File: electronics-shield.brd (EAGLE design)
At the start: 85 x 56 mm, 83 parts, among them IC1 MCP1703CB, Q1 8 MHz, Q2 MOSFET-PCHANNELSMD, U1 TLE9201SGAUMA1, U2 TLE9201SGAUMA1, U3 TLE9201SGAUMA1, U4 TLE9201SGAUMA1, U5 STM32F051C8T, U6 SN74LVC4245APWR, U7 SN74LVC4245APWR, U8 24LC256

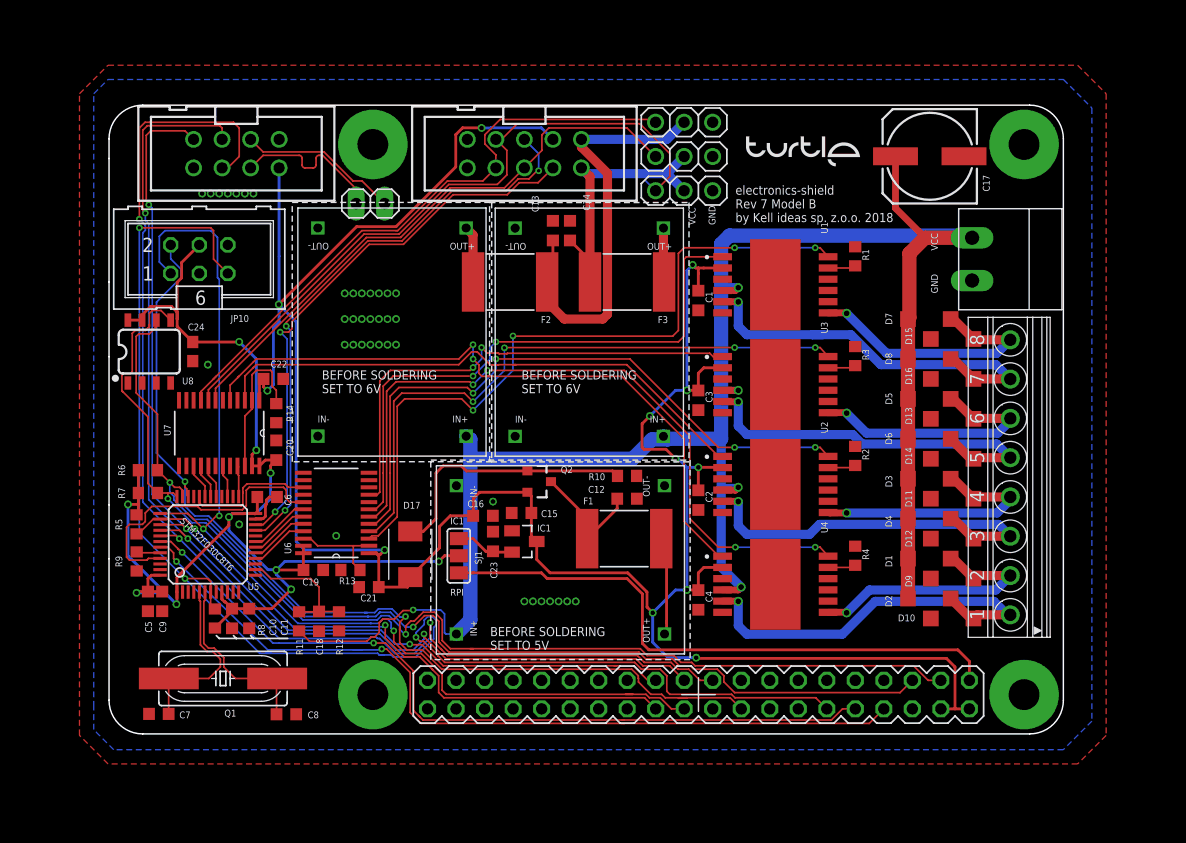
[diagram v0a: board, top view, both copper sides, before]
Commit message: changed base for 7.c
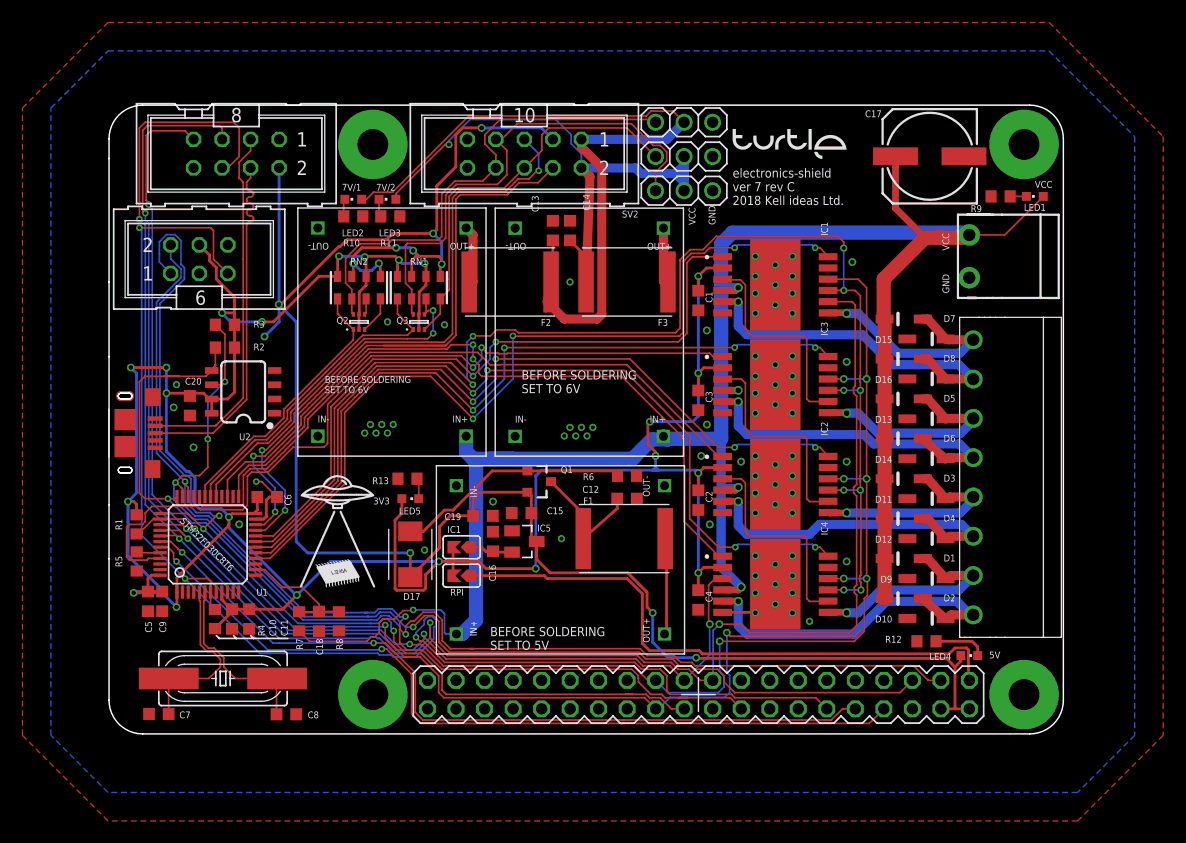
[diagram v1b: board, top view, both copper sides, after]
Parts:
- removed C21, C22, C23: 100n, resistor:C0603K
- removed C24: 0.1uF, rcl:C0603
- removed JP10: gniazdo IDC męskie 6pin proste, con-harting-ml:ML6
- removed JP4: Listwa kołkowa 2.54mm prosta 1x3 (3pin), Synergiczne:1X03
- removed JP5: Listwa stykowa 2.54mm prosta 2x20 (40-pin), wydłużona, RASPBERRY_PI_Bplus-eagle5:2X20
- removed JP6: gniazdo IDC męskie 10pin proste, con-3m:PAK100/2500-10
- removed JP7: gniazdo IDC męskie 8pin proste, Simplex-Connectors:PAK100/2500-10
- removed JP8: Listwa zaciskowa rozłączalna 3.81mm 2pin kątowe 90° gniazdo, con-phoenix-381_l:MC2
- removed JP9: Listwa zaciskowa rozłączalna 3.50mm 8pin kątowe 90° gniazdo, con-phoenix-350:1751303
- removed PCB2, PCB3: Moduł przetwornicy DC-DC Step-down 4.5..28V --- regulowane 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, Kell Ideas:MP1584_MODULE
- removed R14: 10k, resistor:R0603
- removed U5: STM32F051C8T, STM32F030:LQFP48
- removed U6, U7: SN74LVC4245APWR, Texas Instruments_By_element14_Batch_1:SOP65P640X120-24N
- removed U8: 24LC256, SparkFun-IC-Memory:SO08
- added $3_0_$_2018-08-14_21-12-08, $3_1_$_2018-08-14_21-12-08, $3_2_$_2018-08-14_21-12-08: Moduł przetwornicy DC-DC Step-down 4.5..28V --- regulowane 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, Kell Ideas:DC-BRICK
- added IC2: TLE9201SG, Kell Ideas:PG-DSO-12-9
- added IC5: LINEAR_MCP1703CB, electronics-shield:LINEAR_SOT23
- added J1: USB-MICRO-B, Kell Ideas:USB-MICRO-B
- added LED1, LED2, LED3, LED4, LED5: LEDCHIPLED_0603, audio amplifier example:CHIPLED_0603
- added Q3: ON-SEMICONDUCTOR---NTZD3154NT1G_ON_SEMICONDUCTOR_NTZD3154NT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, electronics-shield:ON-SEMICONDUCTOR---NTZD3154NT1G_ON_SEMICONDUCTOR_NTZD3154NT1G_0
- added RN1, RN2: 1k, SparkFun-Resistors:0805-ARV
- added SJ2: (no value), Kell Ideas:SJ
- added SV1: gniazdo IDC męskie 6pin proste, Kell Ideas:ML6
- added SV2: (no value), Kell Ideas:ML10
- added SV3: ML8, Kell Ideas:ML8
- added X1: CONNECTOR_PHOENIX_3.81, Kell Ideas:3.81MM_2PIN
- added X2: Listwa zaciskowa rozłączalna 3.50mm 8pin kątowe 90° gniazdo, Kell Ideas:3.5MM_8PIN
- added Y1: 8 MHz, Kell Ideas:HC49UP
- C1, C10, C11, C12, C13, C14, C15, C16, C18, C19, C2, C3, C4, C5, C6, C7, C8, C9: device resistor:C0603K -> Kell Ideas:C0603K
- C17: device resistor:153CLV-0807 -> Kell Ideas:FI8_6.2
- C20: value 100n -> 0.1uF; device resistor:C0603K -> Kell Ideas:C0603K
- D1, D10, D11, D12, D13, D14, D15, D16, D2, D3, D4, D5, D6, D7, D8, D9: device diode:SOD123 -> Kell Ideas:SOD123
- D17: device diode:SMBJ -> Kell Ideas:SMBJ
- F1, F2, F3: device polyfuse-smd_10:2920L -> Kell Ideas:FUSC7351X125
- IC1: value MCP1703CB -> TLE9201SG; device linear:SOT23 -> Kell Ideas:PG-DSO-12-9
- IC3, IC4: value TLE9201SGAUMA1 -> TLE9201SG
- JP1: value Listwa kołkowa 2.54mm prosta 1x2 (2pin) -> Listwa kołkowa 2.54mm prosta 1x3 (3pin); device pinhead:1X02 -> Kell Ideas:1X03_ROUND_DNP
- JP2, JP3: device Synergiczne:1X03 -> Kell Ideas:1X03_ROUND_DNP
- PCB1: value Moduł przetwornicy DC-DC Step-down 4.5..28V --- regulowane 0.8..20V MP1584 -> Listwa stykowa 2.54mm prosta 2x20 (40-pin), wydłużona; device Kell Ideas:MP1584_MODULE -> Kell Ideas:RASPBERRY_PI_B+_CONNECTOR
- Q1: value 8 MHz -> USER-SUBMITTED_MOSFET-PCHANNELSMD; device crystal:HC49UP -> electronics-shield:USER-SUBMITTED_SOT23-3
- Q2: value MOSFET-PCHANNELSMD -> ON-SEMICONDUCTOR---NTZD3154NT1G_ON_SEMICONDUCTOR_NTZD3154NT1GON_SEMICONDUCTOR_NTZD3154NT1G_0_0; device User-Submitted:SOT23-3 -> electronics-shield:ON-SEMICONDUCTOR---NTZD3154NT1G_ON_SEMICONDUCTOR_NTZD3154NT1G_0
- R1, R4: device rcl:R0603 -> Kell Ideas:R0603
- R10: value 100k -> 330; device rcl:R0603 -> Kell Ideas:R0603
- R11: value 10k -> 330; device resistor:R0603 -> Kell Ideas:R0603
- R12: value 1k -> 200; device resistor:R0603 -> Kell Ideas:R0603
- R13: value 10k -> 200; device resistor:R0603 -> Kell Ideas:R0603
- R2, R3: value 10k -> 4k7; device rcl:R0603 -> Kell Ideas:R0603
- R5: device resistor:R0603 -> Kell Ideas:R0603
- R6: value 4k7 -> 100k; device resistor:R0603 -> Kell Ideas:R0603
- R7: value 4k7 -> 10k; device resistor:R0603 -> Kell Ideas:R0603
- R8: value 10k -> 1k; device resistor:R0603 -> Kell Ideas:R0603
- R9: value 10k -> 1.5k; device resistor:R0603 -> Kell Ideas:R0603
- SJ1: value Zworka cynowa -> (none); device jumper:SJ_2 -> Kell Ideas:SJ
- U1: value TLE9201SGAUMA1 -> STM32F0XX8T; device Kell Ideas:PG-DSO-12-9 -> Kell Ideas:LQFP48
- U2: value TLE9201SGAUMA1 -> EEPROM-I2C; device Kell Ideas:PG-DSO-12-9 -> Kell Ideas:SO-08
- moved R9 83.5 mm to (79.5, 48.0), turned to 180 degrees
- moved PCB1 74.2 mm to (85.1, 56.1), turned to 180 degrees
- moved R1 68.3 mm to (2.54, 18.8), turned to 90 degrees
- moved R4 57.3 mm to (9.53, 10.4)
- moved R2 57.0 mm to (10.4, 34.5), turned to 0 degrees
- moved R3 56.2 mm to (10.4, 36.6), turned to 0 degrees
- moved U1 55.6 mm to (8.89, 17.0), turned to 0 degrees
- moved R12 52.4 mm to (72.9, 8.38), turned to 180 degrees
- moved U2 48.1 mm to (12.0, 30.6), turned to 90 degrees
- moved R6 42.7 mm to (46.2, 23.1)
- moved R11 37.0 mm to (25.1, 46.2), turned to 0 degrees
- moved R10 33.6 mm to (21.8, 46.2), turned to 0 degrees
- moved Q1 33.1 mm to (38.4, 22.6), turned to 270 degrees
- moved IC1 32.0 mm to (59.4, 40.1)
- moved JP1 28.3 mm to (51.3, 51.6)
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- renumbered U3 to IC3, U4 to IC4
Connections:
- removed net EN1_UC: U5.16, U6.21
- removed net EN2_UC: U5.17, U6.20
- removed net EN3_UC: U5.18, U6.19
- removed net EN4_UC: U5.19, U6.18
- removed net IN11_UC: U5.45, U6.17
- removed net IN12: U6.8
- removed net IN12_UC: U6.16
- removed net IN21_UC: U5.32, U6.15
- removed net IN22: U6.10
- removed net IN22_UC: U6.14
- removed net IN31_UC: U5.25, U7.21
- removed net IN32: U7.4
- removed net IN32_UC: U7.20
- removed net IN41_UC: U5.27, U7.19
- removed net IN42: U7.6
- removed net IN42_UC: U7.18
- removed net U5_DIS: R1.2, U1.11
- removed net U6_DIS: R2.2, U2.11
- removed net U7_DIS: IC3.11, R3.2
- removed net U8_DIS: IC4.11, R4.2
- new net N$14: Q2.4, RN2.3
- new net N$16: Q2.3, RN2.4
- new net N$5: LED5.C, R13.1
- new net SO1-SI3: IC1.3, IC3.8
- new net SO2-SI4: IC2.3, IC4.8
- new net SO3-SI2: IC2.8, IC3.3
- new net TLE_NSS: IC1.9, IC2.9, IC3.9, IC4.9, U1.20
- net +3V3: now also C1.1, C2.1, C3.1, C4.1, IC1.2, IC2.2, IC3.2, IC4.2, LED5.A, Q2.2, Q2.5, Q3.2, Q3.5, R1.2, R2.2, R3.2, R4.2, RN1.6, RN1.8, RN2.6, RN2.8, SJ1.1, SJ2.1, SV1.4, U1.1, U1.24, U1.48, U1.9, U2.7, U2.8; no longer C19.1, C24.1, JP10.4, R5.2, R6.2, R7.2, R8.2, SJ1.2, U5.1, U5.24, U5.48, U5.9, U6.23, U6.24, U7.23, U7.24, U8.7, U8.8
- net +5V: now also C19.1, IC5.3, LED4.A, PCB1.2, PCB1.4, Q1.2, RN1.5, RN1.7, RN2.5, RN2.7, SV2.3, SV3.2; no longer C1.1, C2.1, C21.1, C22.1, C23.1, C3.1, C4.1, IC1.3, IC3.2, IC4.2, JP5.2, JP5.4, JP6.3, JP7.2, Q2.2, U1.2, U2.2, U6.1, U7.1
- net +5V_RAW: now also $3_0_$_2018-08-14_21-12-08.OUT1+1; no longer PCB1.OUT1+1
- net +7V/1: now also JP3.2, LED2.A, SV2.1; no longer JP4.2, JP6.1
- net +7V/1_RAW: now also $3_1_$_2018-08-14_21-12-08.OUT1+1; no longer PCB2.OUT1+1
- net +7V/2: now also JP1.2, LED3.A, SV2.2; no longer JP3.2, JP6.2
- net +7V/2_RAW: now also $3_2_$_2018-08-14_21-12-08.OUT1+1; no longer PCB3.OUT1+1
- net 3V3: now also PCB1.17; no longer JP5.17
- net 3V3_RPI: now also PCB1.1, SJ2.2; no longer JP5.1, SJ1.3
- net 3V3_STABILIZED: now also IC5.2, SJ1.2; no longer IC1.2, SJ1.1
- net 5V_NOT_TRIMMED: now also Q1.3; no longer Q2.3
- net BAT_MEAS: now also R7.1, R8.2, U1.14; no longer R11.1, R12.2, U5.14
- net BOOT0: now also R5.2, U1.44; no longer R9.2, U5.44
- net D1-R3: now also Q1.1, R6.2; no longer Q2.1, R10.2
- net DATA_N: now also J1.D-, SV3.3; no longer JP1.2, JP7.3
- net DATA_P: now also J1.D+, SV3.4; no longer JP1.1, JP7.4
- net EN1: now also IC1.12, U1.16; no longer U1.12, U6.3
- net EN2: now also U1.17; no longer U6.4
- net EN3: now also IC2.12, U1.18; no longer U2.12, U6.5
- net EN4: now also U1.19; no longer U6.6
- net GND: now also $3_0_$_2018-08-14_21-12-08.IN1-1, $3_0_$_2018-08-14_21-12-08.OUT1-1, $3_1_$_2018-08-14_21-12-08.IN1-1, $3_1_$_2018-08-14_21-12-08.OUT1-1, $3_2_$_2018-08-14_21-12-08.IN1-1, $3_2_$_2018-08-14_21-12-08.OUT1-1, D10.2, D11.2, D12.2, D13.2, D14.2, D15.2, D16.2, D9.2, IC1.11, IC1.13, IC1.6, IC2.11, IC2.13, IC2.6, IC3.11, IC4.11, IC5.1, J1.GND, J1.SHIELD$1, J1.SHIELD$2, J1.SHIELD$3, J1.SHIELD$4, JP1.3, PCB1.14, PCB1.20, PCB1.25, PCB1.30, PCB1.34, PCB1.39, PCB1.6, PCB1.9, R10.2, R11.2, R12.2, R5.1, R6.1, R8.1, R9.2, SV1.3, SV2.10, SV2.9, SV3.1, SV3.8, U1.23, U1.47, U1.8, U2.2, U2.3, U2.4, X1.1; no longer C21.2, C22.2, C23.2, C24.2, D10.A, D11.A, D12.A, D13.A, D14.A, D15.A, D16.A, D9.A, IC1.1, JP10.3, JP4.3, JP5.14, JP5.20, JP5.25, JP5.30, JP5.34, JP5.39, JP5.6, JP5.9, JP6.10, JP6.9, JP7.1, JP7.8, JP8.1, PCB1.IN1-1, PCB1.OUT1-1, PCB2.IN1-1, PCB2.OUT1-1, PCB3.IN1-1, PCB3.OUT1-1, R1.1, R10.1, R12.1, R14.2, R2.1, R3.1, R4.1, R9.1, U1.13, U1.6, U2.13, U2.6, U5.23, U5.47, U5.8, U6.11, U6.12, U6.13, U7.11, U7.12, U7.13, U8.2, U8.3, U8.4
- net IN11: now also IC1.1, U1.45; no longer U1.1, U6.7
- net IN21: now also U1.32; no longer U6.9
- net IN31: now also IC2.1, U1.25; no longer U2.1, U7.3
- net IN41: now also U1.27; no longer U7.5
- net LED: now also U1.15; no longer U5.15
- net MOT11: now also D16.1, D8.2, IC1.5, X2.7; no longer D16.C, D8.A, JP9.7, U1.5
- net MOT12: now also D15.1, D7.2, IC1.7, X2.8; no longer D15.C, D7.A, JP9.8, U1.7
- net MOT21: now also D14.1, D6.2, X2.5; no longer D14.C, D6.A, JP9.5
- net MOT22: now also D13.1, D5.2, X2.6; no longer D13.C, D5.A, JP9.6
- net MOT31: now also D12.1, D4.2, IC2.5, X2.3; no longer D12.C, D4.A, JP9.3, U2.5
- net MOT32: now also D11.1, D3.2, IC2.7, X2.4; no longer D11.C, D3.A, JP9.4, U2.7
- net MOT41: now also D10.1, D2.2, X2.1; no longer D10.C, D2.A, JP9.1
- net MOT42: now also D1.2, D9.1, X2.2; no longer D1.A, D9.C, JP9.2
- net N$1: now also LED1.C, R9.1; no longer R13.1, U6.2, U6.22
- net N$2: now also LED2.C, R10.1; no longer R14.1, U7.2, U7.22
- net N$3: now also LED3.C, R11.1; no longer U7.10
- net N$4: now also LED4.C, R12.1; no longer U7.14
- net N$8: now also SV1.6; no longer JP10.6
- net NRST: now also PCB1.12, R4.1, SV1.5, U1.7; no longer JP10.5, JP5.12, R8.1, U5.7
- net OSCILATOR_N: now also U1.5, Y1.2; no longer Q1.2, U5.5
- net OSCILATOR_P: now also U1.6, Y1.1; no longer Q1.1, U5.6
- net RPI_CLK: now also IC1.10, IC2.10, IC3.10, IC4.10, PCB1.23, SV3.7, U1.39; no longer JP5.23, JP7.7, U5.39
- net RPI_MISO: now also IC4.3, PCB1.21, SV3.5, U1.40; no longer JP5.21, JP7.5, U5.40
- net RPI_MOSI: now also IC1.8, PCB1.19, SV3.6, U1.41; no longer JP5.19, JP7.6, U5.41
- net RPI_RXD: now also PCB1.10, U1.42; no longer JP5.10, U5.42
- net RPI_TXD: now also PCB1.8, U1.43; no longer JP5.8, U5.43
- net SCL: now also PCB1.5, R3.1, U1.35, U2.6; no longer JP5.5, R7.1, U5.35, U8.6
- net SCL_TX: now also SV2.5, U1.21; no longer JP6.5, U5.21
- net SDA: now also PCB1.3, R2.1, U1.36, U2.5; no longer JP5.3, R6.1, U5.36, U8.5
- net SDA_RX: now also SV2.4, U1.22; no longer JP6.4, U5.22
- net SEN1: now also U1.10; no longer U5.10
- net SEN2: now also U1.11; no longer U5.11
- net SEN3: now also U1.12; no longer U5.12
- net SEN4: now also U1.13; no longer U5.13
- net SERVO1: now also JP1.1, Q3.3, RN1.4, SV2.6; no longer JP2.1, JP6.6, U7.7
- net SERVO1_UC: now also Q3.4, RN1.3, U1.29; no longer U5.29, U7.17
- net SERVO2: now also JP2.1, Q3.6, RN1.2, SV2.7; no longer JP3.1, JP6.7, U7.8
- net SERVO2_UC: now also Q3.1, RN1.1, U1.30; no longer U5.30, U7.16
- net SERVO3: now also JP3.1, Q2.6, RN2.2, SV2.8; no longer JP4.1, JP6.8, U7.9
- net SERVO3_UC: now also Q2.1, RN2.1, U1.31; no longer U5.31, U7.15
- net SPI1_NSS: now also PCB1.24, R1.1, U1.38; no longer JP5.24, R5.1, U5.38
- net SWCLK: now also PCB1.22, SV1.1, U1.37; no longer JP10.1, JP5.22, U5.37
- net SWDIO: now also PCB1.18, SV1.2, U1.34; no longer JP10.2, JP5.18, U5.34
- net VCC: now also $3_0_$_2018-08-14_21-12-08.IN1+1, $3_1_$_2018-08-14_21-12-08.IN1+1, $3_2_$_2018-08-14_21-12-08.IN1+1, D1.1, D2.1, D3.1, D4.1, D5.1, D6.1, D7.1, D8.1, IC1.4, IC2.4, LED1.A, R7.2, X1.2; no longer D1.C, D2.C, D3.C, D4.C, D5.C, D6.C, D7.C, D8.C, JP8.2, PCB1.IN1+1, PCB2.IN1+1, PCB3.IN1+1, R11.2, U1.4, U2.4
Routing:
- net +3V3: track 119.9 -> 258.0 mm, vias 10 -> 22
- net TLE_NSS: track 0.00 -> 118.1 mm, vias 0 -> 10
- net RPI_CLK: track 91.2 -> 160.1 mm, vias 3 -> 10
- net RPI_MOSI: track 110.6 -> 160.1 mm, vias 3 -> 4
- net +5V: track 225.1 -> 180.3 mm
- net +7V/1: track 38.2 -> 69.7 mm
- net +7V/2: track 27.1 -> 56.0 mm, vias 0 -> 1
- net SERVO1_UC: track 3.02 -> 30.8 mm, vias 0 -> 2
- net IN11: track 51.5 -> 78.6 mm
- net IN11_UC: track 26.2 -> 0.00 mm
- net SERVO2_UC: track 3.09 -> 28.6 mm
- net SPI1_NSS: track 55.6 -> 80.4 mm, vias 2 -> 3
- net SERVO3_UC: track 3.16 -> 24.3 mm
- net SO1-SI3: track 0.00 -> 20.1 mm
- net SO2-SI4: track 0.00 -> 19.6 mm
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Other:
- board text added: "3V3"
- board text added: "5V"
- board text added: "7V/1"
- board text added: "7V/2"
- board text added: "electronics-shield ver 7 rev C 2018 Kell ideas Ltd."
- board text removed: "electronics-shield Rev 7 Model B by Kell ideas sp. z.o.o. 2018"
